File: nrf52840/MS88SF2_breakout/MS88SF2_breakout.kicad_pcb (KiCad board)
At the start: 2 copper layers, 3 parts, among them J1 Conn_01x14_Male, J2 Conn_01x14_Male, U1 MS88SF2

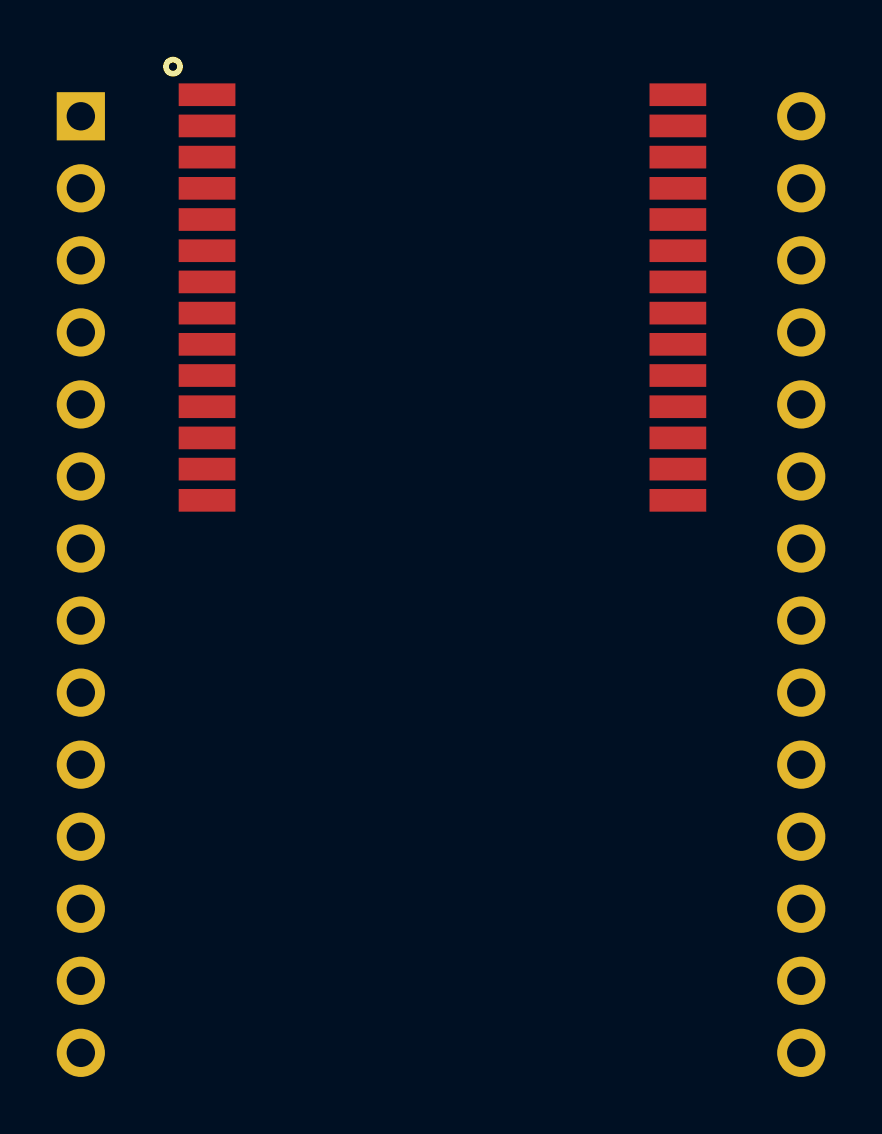
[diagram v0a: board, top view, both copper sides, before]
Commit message: nrf5: Prepare for routing
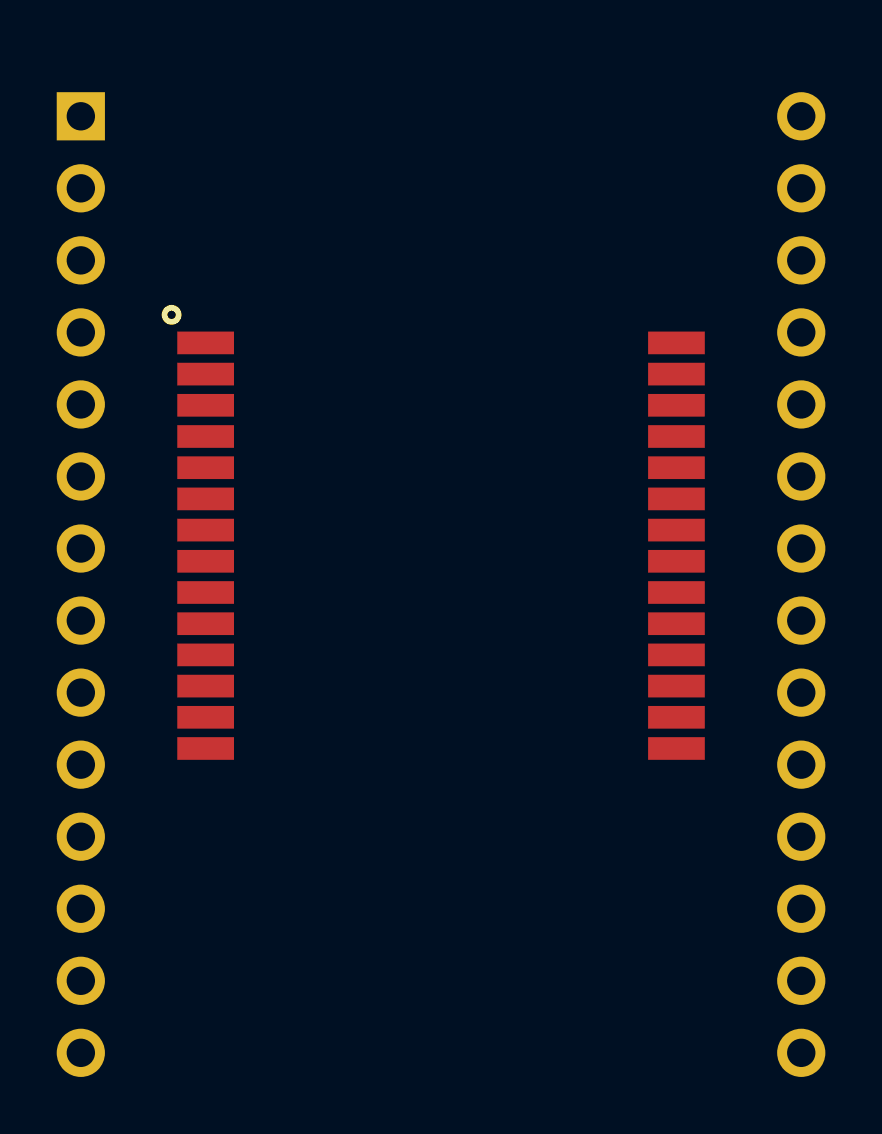
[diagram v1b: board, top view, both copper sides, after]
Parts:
- moved U1 8.75 mm to (75.7, 72.0)
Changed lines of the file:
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@@
     (thickness 1.6)
     (drawings 0)
-    (tracks 1)
+    (tracks 0)
     (zones 0)
     (modules 3)
@@
     (47 F.CrtYd user)
     (48 B.Fab user)
-    (49 F.Fab user hide)
+    (49 F.Fab user)
   )
   (setup
-    (last_trace_width 0.8)
+    (last_trace_width 0.4)
     (user_trace_width 0.4)
     (user_trace_width 0.8)
@@
   )
   (module MS88SF2:MS88SF2 (layer F.Cu)
-    (at 75.75 63.25)
+    (at 75.7 72)
     (fp_text reference U1 (at 8 12.5) (layer F.Fab)
       (effects (font (size 1 1) (thickness 0.15)))
@@
       (effects (font (size 1 1) (thickness 0.15)))
     )
+    (fp_line (start -12.7 -5.81) (end 12.7 -17.6) (layer F.Fab) (width 0.12))
+    (fp_line (start 12.7 -5.81) (end -12.7 -17.6) (layer F.Fab) (width 0.12))
+    (fp_circle (center -9.5 -5) (end -9.4 -5) (layer F.SilkS) (width 0.5))
+    (fp_line (start 12.7 -17.6) (end -12.7 -17.6) (layer F.Fab) (width 0.12))
+    (fp_line (start 8.7 -5.81) (end -8.7 -5.81) (layer F.Fab) (width 0.12))
+    (fp_line (start 12.7 -5.81) (end 12.7 -17.6) (layer F.Fab) (width 0.12))
+    (fp_line (start 8.7 -5.81) (end 12.7 -5.81) (layer F.Fab) (width 0.12))
+    (fp_line (start -12.7 -5.81) (end -12.7 -17.6) (layer F.Fab) (width 0.12))
+    (fp_line (start -8.7 -5.81) (end -12.7 -5.81) (layer F.Fab) (width 0.12))
+    (fp_line (start 8.7 11.6) (end 8.7 -11.6) (layer F.Fab) (width 0.12))
+    (fp_line (start -8.7 11.6) (end 8.7 11.6) (layer F.Fab) (width 0.12))
+    (fp_line (start -8.7 -11.6) (end -8.7 11.6) (layer F.Fab) (width 0.12))
+    (fp_line (start 8.7 -11.6) (end -8.7 -11.6) (layer F.Fab) (width 0.12))
     (fp_text user "No copper" (at 0 -16) (layer F.Fab)
       (effects (font (size 1 1) (thickness 0.15)))
     )
-    (fp_line (start 8.7 -11.6) (end -8.7 -11.6) (layer F.Fab) (width 0.12))
-    (fp_line (start -8.7 -11.6) (end -8.7 11.6) (layer F.Fab) (width 0.12))
-    (fp_line (start -8.7 11.6) (end 8.7 11.6) (layer F.Fab) (width 0.12))
-    (fp_line (start 8.7 11.6) (end 8.7 -11.6) (layer F.Fab) (width 0.12))
-    (fp_line (start -8.7 -5.81) (end -12.7 -5.81) (layer F.Fab) (width 0.12))
-    (fp_line (start -12.7 -5.81) (end -12.7 -17.6) (layer F.Fab) (width 0.12))
-    (fp_line (start 8.7 -5.81) (end 12.7 -5.81) (layer F.Fab) (width 0.12))
-    (fp_line (start 12.7 -5.81) (end 12.7 -17.6) (layer F.Fab) (width 0.12))
-    (fp_line (start 8.7 -5.81) (end -8.7 -5.81) (layer F.Fab) (width 0.12))
-    (fp_line (start 12.7 -17.6) (end -12.7 -17.6) (layer F.Fab) (width 0.12))
-    (fp_circle (center -9.5 -5) (end -9.4 -5) (layer F.SilkS) (width 0.5))
-    (fp_line (start 12.7 -5.81) (end -12.7 -17.6) (layer F.Fab) (width 0.12))
-    (fp_line (start -12.7 -5.81) (end 12.7 -17.6) (layer F.Fab) (width 0.12))
     (pad 1 smd rect (at -8.3 -4.01) (size 2 0.8) (layers F.Cu F.Paste F.Mask)
       (net 2 GND))
@@
       (effects (font (size 1 1) (thickness 0.15)))
     )
+    (fp_line (start -1.27 -0.635) (end -0.635 -1.27) (layer F.Fab) (width 0.1))
+    (fp_line (start -1.27 34.29) (end -1.27 -0.635) (layer F.Fab) (width 0.1))
+    (fp_line (start 1.27 34.29) (end -1.27 34.29) (layer F.Fab) (width 0.1))
+    (fp_line (start 1.27 -1.27) (end 1.27 34.29) (layer F.Fab) (width 0.1))
+    (fp_line (start -0.635 -1.27) (end 1.27 -1.27) (layer F.Fab) (width 0.1))
     (fp_text user %R (at 0 16.51 90) (layer F.Fab)
       (effects (font (size 1 1) (thickness 0.15)))
     )
-    (fp_line (start -0.635 -1.27) (end 1.27 -1.27) (layer F.Fab) (width 0.1))
-    (fp_line (start 1.27 -1.27) (end 1.27 34.29) (layer F.Fab) (width 0.1))
-    (fp_line (start 1.27 34.29) (end -1.27 34.29) (layer F.Fab) (width 0.1))
-    (fp_line (start -1.27 34.29) (end -1.27 -0.635) (layer F.Fab) (width 0.1))
-    (fp_line (start -1.27 -0.635) (end -0.635 -1.27) (layer F.Fab) (width 0.1))
     (pad 14 thru_hole oval (at 0 33.02) (size 1.7 1.7) (drill 1) (layers *.Cu *.Mask)
       (net 1 +3V3))
@@
       (effects (font (size 1 1) (thickness 0.15)))
     )
+    (fp_line (start -0.635 -1.27) (end 1.27 -1.27) (layer F.Fab) (width 0.1))
+    (fp_line (start 1.27 -1.27) (end 1.27 34.29) (layer F.Fab) (width 0.1))
+    (fp_line (start 1.27 34.29) (end -1.27 34.29) (layer F.Fab) (width 0.1))
+    (fp_line (start -1.27 34.29) (end -1.27 -0.635) (layer F.Fab) (width 0.1))
+    (fp_line (start -1.27 -0.635) (end -0.635 -1.27) (layer F.Fab) (width 0.1))
     (fp_text user %R (at 0 16.51 90) (layer F.Fab)
       (effects (font (size 1 1) (thickness 0.15)))
     )
-    (fp_line (start -1.27 -0.635) (end -0.635 -1.27) (layer F.Fab) (width 0.1))
-    (fp_line (start -1.27 34.29) (end -1.27 -0.635) (layer F.Fab) (width 0.1))
-    (fp_line (start 1.27 34.29) (end -1.27 34.29) (layer F.Fab) (width 0.1))
-    (fp_line (start 1.27 -1.27) (end 1.27 34.29) (layer F.Fab) (width 0.1))
-    (fp_line (start -0.635 -1.27) (end 1.27 -1.27) (layer F.Fab) (width 0.1))
     (pad 15 thru_hole oval (at 0 33.02) (size 1.7 1.7) (drill 1) (layers *.Cu *.Mask))
     (pad 16 thru_hole oval (at 0 30.48) (size 1.7 1.7) (drill 1) (layers *.Cu *.Mask))
@@
     )
   )
-  (segment (start 63.45 62.54) (end 63 62.54) (width 0.8) (layer F.Cu) (net 24))
 )

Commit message: nrf5: Adjust position
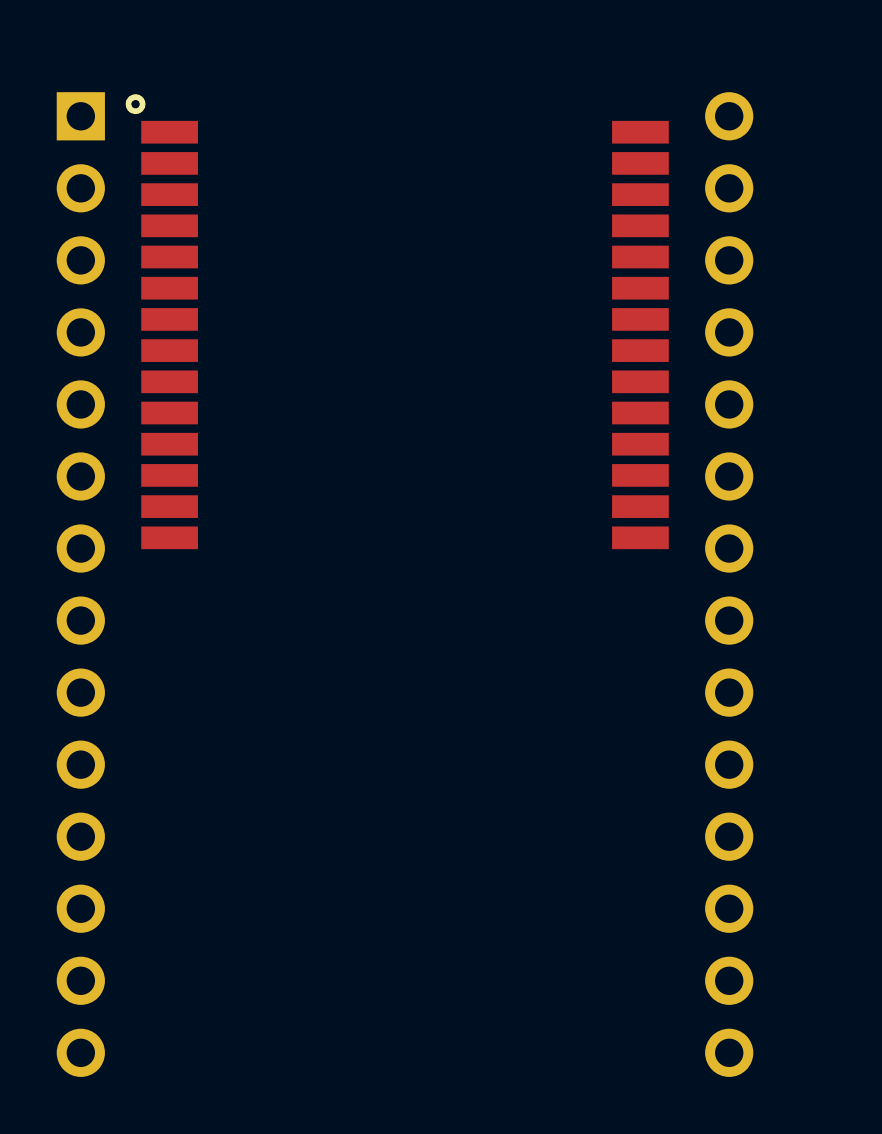
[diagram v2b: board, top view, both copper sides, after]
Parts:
- moved U1 7.54 mm to (74.4, 64.6)
- moved J2 2.54 mm to (85.9, 60.0)
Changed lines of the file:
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@@
   )
   (setup
-    (last_trace_width 0.4)
+    (last_trace_width 0.25)
     (user_trace_width 0.4)
     (user_trace_width 0.8)
@@
   )
   (module MS88SF2:MS88SF2 (layer F.Cu)
-    (at 75.7 72)
+    (at 74.43 64.572)
     (fp_text reference U1 (at 8 12.5) (layer F.Fab)
       (effects (font (size 1 1) (thickness 0.15)))
@@
       (effects (font (size 1 1) (thickness 0.15)))
     )
+    (fp_line (start 8.7 -11.6) (end -8.7 -11.6) (layer F.Fab) (width 0.12))
+    (fp_line (start -8.7 -11.6) (end -8.7 11.6) (layer F.Fab) (width 0.12))
+    (fp_line (start -8.7 11.6) (end 8.7 11.6) (layer F.Fab) (width 0.12))
+    (fp_line (start 8.7 11.6) (end 8.7 -11.6) (layer F.Fab) (width 0.12))
+    (fp_line (start -8.7 -5.81) (end -12.7 -5.81) (layer F.Fab) (width 0.12))
+    (fp_line (start -12.7 -5.81) (end -12.7 -17.6) (layer F.Fab) (width 0.12))
+    (fp_line (start 8.7 -5.81) (end 12.7 -5.81) (layer F.Fab) (width 0.12))
+    (fp_line (start 12.7 -5.81) (end 12.7 -17.6) (layer F.Fab) (width 0.12))
+    (fp_line (start 8.7 -5.81) (end -8.7 -5.81) (layer F.Fab) (width 0.12))
+    (fp_line (start 12.7 -17.6) (end -12.7 -17.6) (layer F.Fab) (width 0.12))
+    (fp_circle (center -9.5 -5) (end -9.4 -5) (layer F.SilkS) (width 0.5))
+    (fp_line (start 12.7 -5.81) (end -12.7 -17.6) (layer F.Fab) (width 0.12))
     (fp_line (start -12.7 -5.81) (end 12.7 -17.6) (layer F.Fab) (width 0.12))
-    (fp_line (start 12.7 -5.81) (end -12.7 -17.6) (layer F.Fab) (width 0.12))
-    (fp_circle (center -9.5 -5) (end -9.4 -5) (layer F.SilkS) (width 0.5))
-    (fp_line (start 12.7 -17.6) (end -12.7 -17.6) (layer F.Fab) (width 0.12))
-    (fp_line (start 8.7 -5.81) (end -8.7 -5.81) (layer F.Fab) (width 0.12))
-    (fp_line (start 12.7 -5.81) (end 12.7 -17.6) (layer F.Fab) (width 0.12))
-    (fp_line (start 8.7 -5.81) (end 12.7 -5.81) (layer F.Fab) (width 0.12))
-    (fp_line (start -12.7 -5.81) (end -12.7 -17.6) (layer F.Fab) (width 0.12))
-    (fp_line (start -8.7 -5.81) (end -12.7 -5.81) (layer F.Fab) (width 0.12))
-    (fp_line (start 8.7 11.6) (end 8.7 -11.6) (layer F.Fab) (width 0.12))
-    (fp_line (start -8.7 11.6) (end 8.7 11.6) (layer F.Fab) (width 0.12))
-    (fp_line (start -8.7 -11.6) (end -8.7 11.6) (layer F.Fab) (width 0.12))
-    (fp_line (start 8.7 -11.6) (end -8.7 -11.6) (layer F.Fab) (width 0.12))
     (fp_text user "No copper" (at 0 -16) (layer F.Fab)
       (effects (font (size 1 1) (thickness 0.15)))
@@
       (net 3 P0.10))
   )
-  (module !myfoots:PinHeader_1x14_P2.54mm_Vertical locked (layer F.Cu)
+  (module !myfoots:PinHeader_1x14_P2.54mm_Vertical (layer F.Cu)
     (at 63 60)
     (descr "Through hole straight pin header, 1x14, 2.54mm pitch, single row")
@@
       (effects (font (size 1 1) (thickness 0.15)))
     )
+    (fp_line (start -0.635 -1.27) (end 1.27 -1.27) (layer F.Fab) (width 0.1))
+    (fp_line (start 1.27 -1.27) (end 1.27 34.29) (layer F.Fab) (width 0.1))
+    (fp_line (start 1.27 34.29) (end -1.27 34.29) (layer F.Fab) (width 0.1))
+    (fp_line (start -1.27 34.29) (end -1.27 -0.635) (layer F.Fab) (width 0.1))
     (fp_line (start -1.27 -0.635) (end -0.635 -1.27) (layer F.Fab) (width 0.1))
-    (fp_line (start -1.27 34.29) (end -1.27 -0.635) (layer F.Fab) (width 0.1))
-    (fp_line (start 1.27 34.29) (end -1.27 34.29) (layer F.Fab) (width 0.1))
-    (fp_line (start 1.27 -1.27) (end 1.27 34.29) (layer F.Fab) (width 0.1))
-    (fp_line (start -0.635 -1.27) (end 1.27 -1.27) (layer F.Fab) (width 0.1))
     (fp_text user %R (at 0 16.51 90) (layer F.Fab)
       (effects (font (size 1 1) (thickness 0.15)))
@@
     )
   )
-  (module !myfoots:PinHeader_1x14_P2.54mm_Vertical_2row locked (layer F.Cu)
-    (at 88.4 60)
+  (module !myfoots:PinHeader_1x14_P2.54mm_Vertical_2row (layer F.Cu)
+    (at 85.86 60)
     (descr "Through hole straight pin header, 1x14, 2.54mm pitch, single row")
     (tags "Through hole pin header THT 1x14 2.54mm single row")
@@
       (effects (font (size 1 1) (thickness 0.15)))
     )
+    (fp_line (start -1.27 -0.635) (end -0.635 -1.27) (layer F.Fab) (width 0.1))
+    (fp_line (start -1.27 34.29) (end -1.27 -0.635) (layer F.Fab) (width 0.1))
+    (fp_line (start 1.27 34.29) (end -1.27 34.29) (layer F.Fab) (width 0.1))
+    (fp_line (start 1.27 -1.27) (end 1.27 34.29) (layer F.Fab) (width 0.1))
     (fp_line (start -0.635 -1.27) (end 1.27 -1.27) (layer F.Fab) (width 0.1))
-    (fp_line (start 1.27 -1.27) (end 1.27 34.29) (layer F.Fab) (width 0.1))
-    (fp_line (start 1.27 34.29) (end -1.27 34.29) (layer F.Fab) (width 0.1))
-    (fp_line (start -1.27 34.29) (end -1.27 -0.635) (layer F.Fab) (width 0.1))
-    (fp_line (start -1.27 -0.635) (end -0.635 -1.27) (layer F.Fab) (width 0.1))
     (fp_text user %R (at 0 16.51 90) (layer F.Fab)
       (effects (font (size 1 1) (thickness 0.15)))
